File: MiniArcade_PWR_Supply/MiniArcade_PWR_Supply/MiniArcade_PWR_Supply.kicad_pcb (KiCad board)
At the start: 2 copper layers, 53.5 x 55.2 mm, 17 parts, among them IC1 MIC94310-SYM5-TR, J1 Conn_01x03, J2 Conn_01x02_Pin, J3 Conn_01x02_Pin, U1 2479

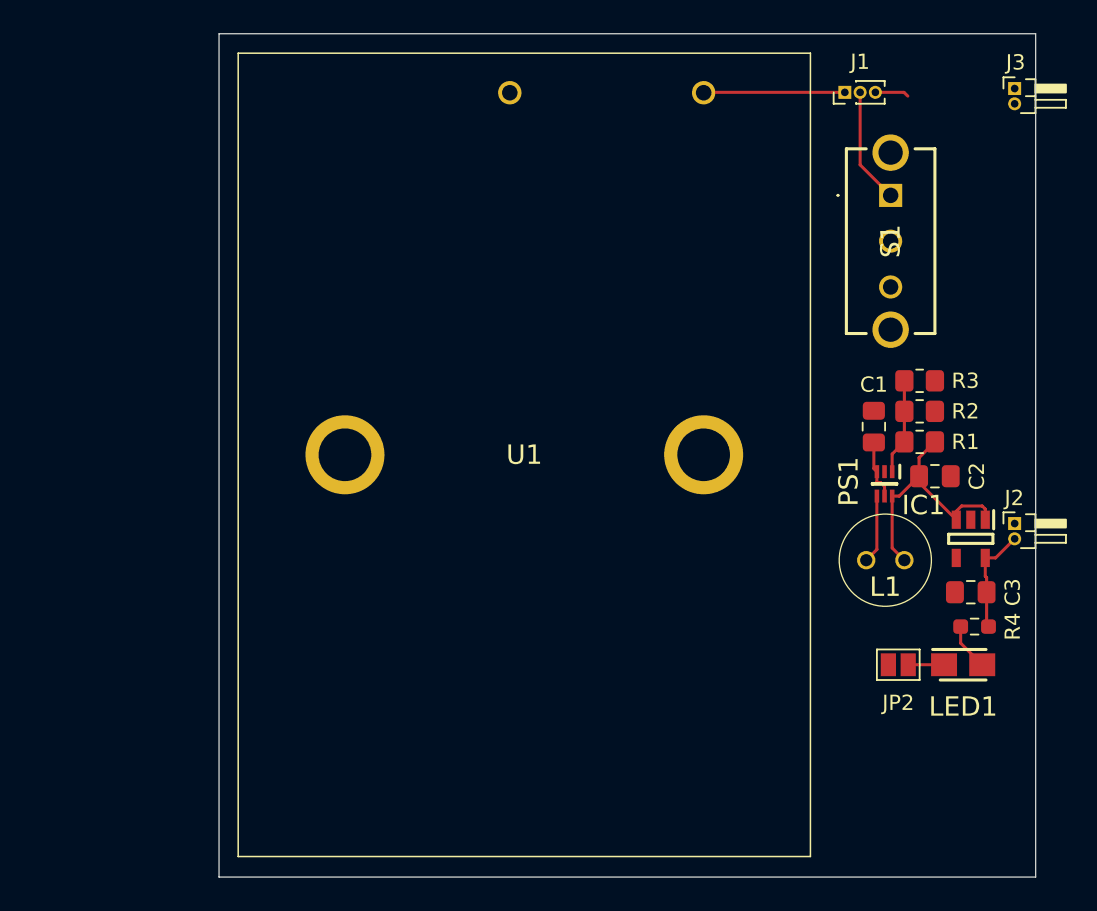
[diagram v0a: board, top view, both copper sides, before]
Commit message: 05 11 2025
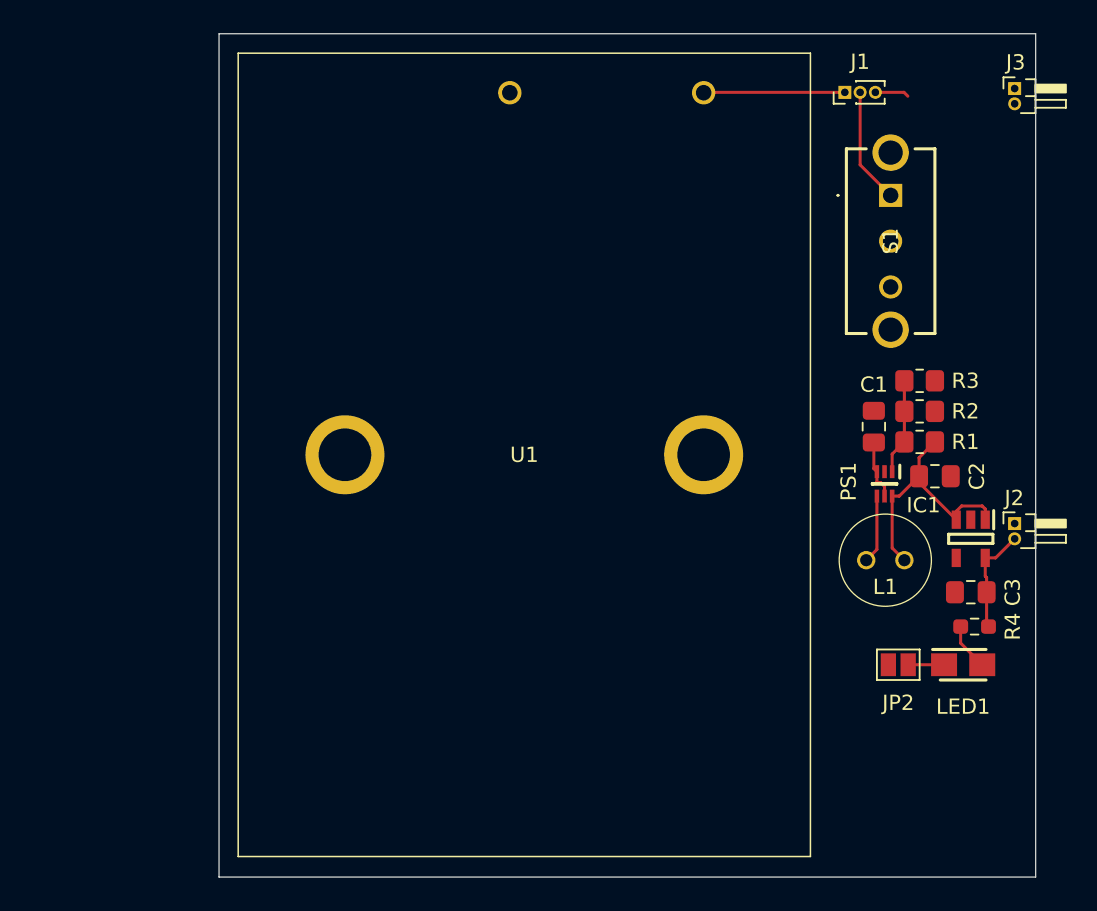
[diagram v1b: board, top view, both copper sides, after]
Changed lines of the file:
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@@
 			(effects
 				(font
-					(size 0.5 0.5)
-					(thickness 0.08)
+					(size 1 1)
+					(thickness 0.15)
 				)
 			)
@@
 			(effects
 				(font
-					(size 1.27 1.27)
-					(thickness 0.254)
+					(size 1 1)
+					(thickness 0.15)
 				)
 			)
@@
 			(effects
 				(font
-					(size 1.27 1.27)
-					(thickness 0.254)
+					(size 1 1)
+					(thickness 0.15)
 				)
 			)
@@
 			(effects
 				(font
-					(size 0.5 0.5)
-					(thickness 0.08)
+					(size 1 1)
+					(thickness 0.15)
 				)
 			)
@@
 			(effects
 				(font
-					(size 1.27 1.27)
-					(thickness 0.254)
+					(size 1 1)
+					(thickness 0.15)
 				)
 			)
@@
 			(effects
 				(font
-					(size 1.27 1.27)
-					(thickness 0.254)
+					(size 1 1)
+					(thickness 0.15)
 				)
 			)
@@
 			(effects
 				(font
-					(size 0.6 0.6)
-					(thickness 0.09)
+					(size 1 1)
+					(thickness 0.15)
 				)
 			)
@@
 			(effects
 				(font
-					(size 1.27 1.27)
-					(thickness 0.254)
+					(size 1 1)
+					(thickness 0.15)
 				)
 			)
@@
 			(effects
 				(font
-					(size 1.27 1.27)
-					(thickness 0.254)
+					(size 1 1)
+					(thickness 0.15)
 				)
 			)
@@
 			(effects
 				(font
-					(size 1.27 1.27)
-					(thickness 0.254)
+					(size 1 1)
+					(thickness 0.15)
 				)
 			)
@@
 			(effects
 				(font
-					(size 1.27 1.27)
-					(thickness 0.254)
+					(size 1 1)
+					(thickness 0.15)
 				)
 			)
@@
 			(effects
 				(font
-					(size 0.6 0.6)
-					(thickness 0.09)
+					(size 1 1)
+					(thickness 0.15)
 				)
 			)
@@
 			(effects
 				(font
-					(size 0.5 0.5)
-					(thickness 0.08)
+					(size 1 1)
+					(thickness 0.15)
 				)
 			)
@@
 			(effects
 				(font
-					(size 0.5 0.5)
-					(thickness 0.08)
+					(size 1 1)
+					(thickness 0.15)
 				)
 			)
@@
 			(effects
 				(font
-					(size 0.76 0.76)
-					(thickness 0.114)
+					(size 1 1)
+					(thickness 0.15)
 				)
 			)
@@
 			(effects
 				(font
-					(size 0.5 0.5)
-					(thickness 0.08)
+					(size 1 1)
+					(thickness 0.15)
 				)
 			)
@@
 			(effects
 				(font
-					(size 1.27 1.27)
-					(thickness 0.254)
+					(size 1 1)
+					(thickness 0.15)
 				)
 			)
@@
 			(effects
 				(font
-					(size 1.27 1.27)
-					(thickness 0.254)
+					(size 1 1)
+					(thickness 0.15)
 				)
 			)
@@
 			(effects
 				(font
-					(size 0.4 0.4)
-					(thickness 0.06)
+					(size 1 1)
+					(thickness 0.15)
 				)
 			)
@@
 			(effects
 				(font
-					(size 1.27 1.27)
-					(thickness 0.254)
+					(size 1 1)
+					(thickness 0.15)
 				)
 			)
@@
 			(effects
 				(font
-					(size 1.27 1.27)
-					(thickness 0.254)
+					(size 1 1)
+					(thickness 0.15)
 				)
 			)
@@
 			(effects
 				(font
-					(size 0.5 0.5)
-					(thickness 0.08)
+					(size 1 1)
+					(thickness 0.15)
 				)
 			)

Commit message: 10 11 2025
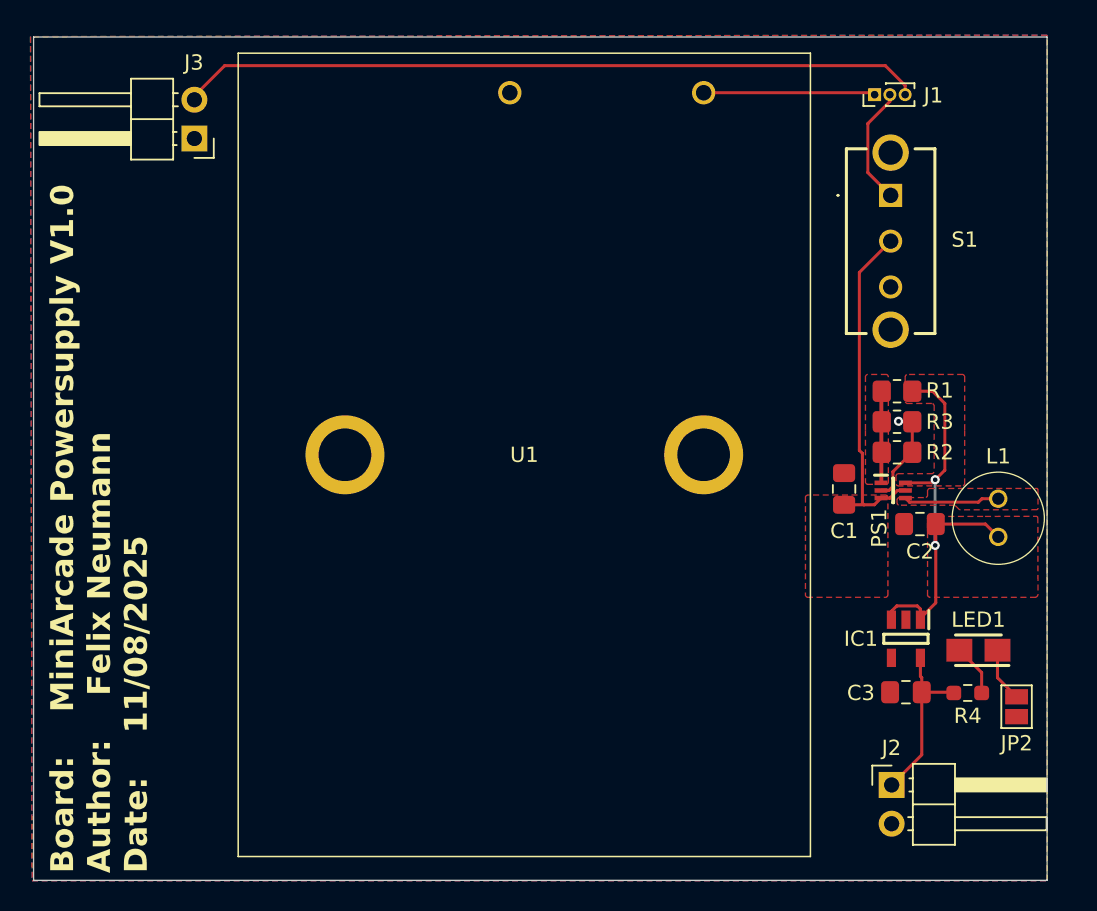
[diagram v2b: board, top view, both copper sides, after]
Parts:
- J2, J3: footprint Connector_PinHeader_1.00mm:PinHeader_1x02_P1.00mm_Horizontal -> Connector_PinHeader_2.54mm:PinHeader_1x02_P2.54mm_Horizontal
- moved J3 53.8 mm to (146.1, 49.3), turned to 180 degrees
- moved J2 18.9 mm to (191.8, 91.6)
- moved JP2 8.22 mm to (200.0, 86.5), turned to 90 degrees
- moved L1 7.90 mm to (198.8, 74.1), turned to -90 degrees
- moved C3 7.81 mm to (192.8, 85.5)
- moved IC1 7.81 mm to (192.8, 82.0)
- moved C1 4.52 mm to (188.7, 72.2)
- moved R4 4.37 mm to (196.8, 85.6), turned to 0 degrees
- moved R1 3.63 mm to (192.2, 65.8)
- moved C2 3.28 mm to (193.7, 74.5), turned to 180 degrees
- moved R2 3.06 mm to (192.2, 69.8)
- moved R3 3.06 mm to (192.2, 67.8)
- moved J1 1.96 mm to (190.7, 46.4)
- moved LED1 1.38 mm to (197.5, 82.8), turned to 180 degrees
- moved PS1 0.71 mm to (191.9, 72.3), turned to 0 degrees
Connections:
- J2 pad 1: GND -> 3V3
- J2 pad 2: 3V3 -> GND
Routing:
- net 5V0: track 2.23 -> 48.9 mm
- net Net-(PS1-EN): track 3.92 -> 22.6 mm
- net 3V5: track 16.8 -> 30.1 mm, vias 0 -> 2
- net GND: track 0.00 -> 6.56 mm, vias 0 -> 1
- net Net-(PS1-FB): track 6.28 -> 12.0 mm
- net 3V3: track 7.03 -> 11.6 mm
- net 4V5: track 9.27 -> 11.3 mm
- net Net-(PS1-SW): track 4.49 -> 6.29 mm
- net Net-(JP2-B): track 2.35 -> 3.57 mm
- added copper zone on F.Cu, net 3V5
- added copper zone on B.Cu, net GND
- added copper zone on F.Cu, net GND
- added copper zone on F.Cu, net Net-(PS1-EN)
- added copper zone on F.Cu, net Net-(PS1-FB)
- added copper zone on F.Cu, net Net-(PS1-SW)
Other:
- board size 53.5 x 55.2 mm -> 66.4 x 55.2 mm
- board text added: "Board: MiniArcade Powersupply V1.0 Author: Felix Neumann Date: 11/08/2025"
